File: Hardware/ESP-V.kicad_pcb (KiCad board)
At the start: 2 copper layers, 23.2 x 37.4 mm, 43 parts, among them J1 USB_C_Receptacle_USB2.0, J2 Conn_01x16_Male, J3 Conn_01x14_Female, J4 USB_A, U1 CH552E, U2 AP7333-33SRG-7, U3 AP7333-33SRG-7, U4 ESP32-C3, Y1 40MHz, Y2 32k

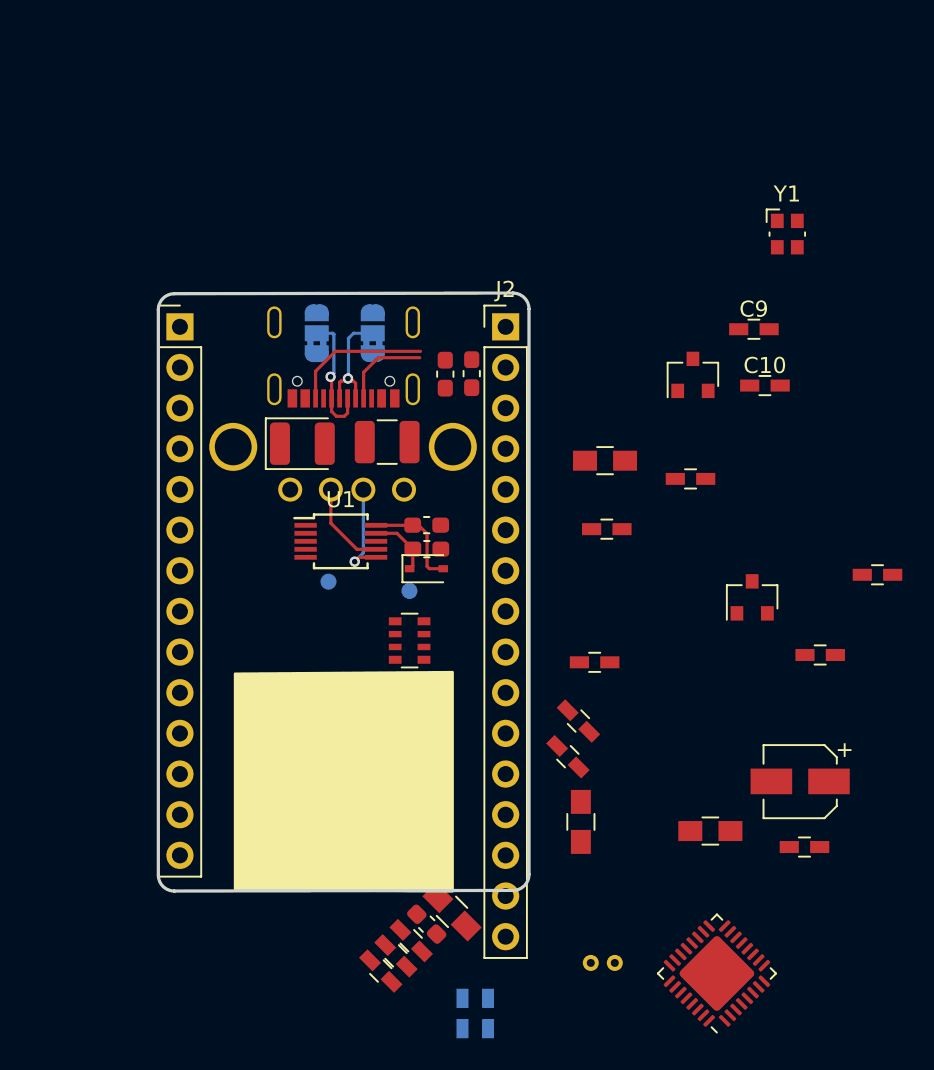
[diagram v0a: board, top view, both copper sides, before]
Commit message: v1.1 ready to order
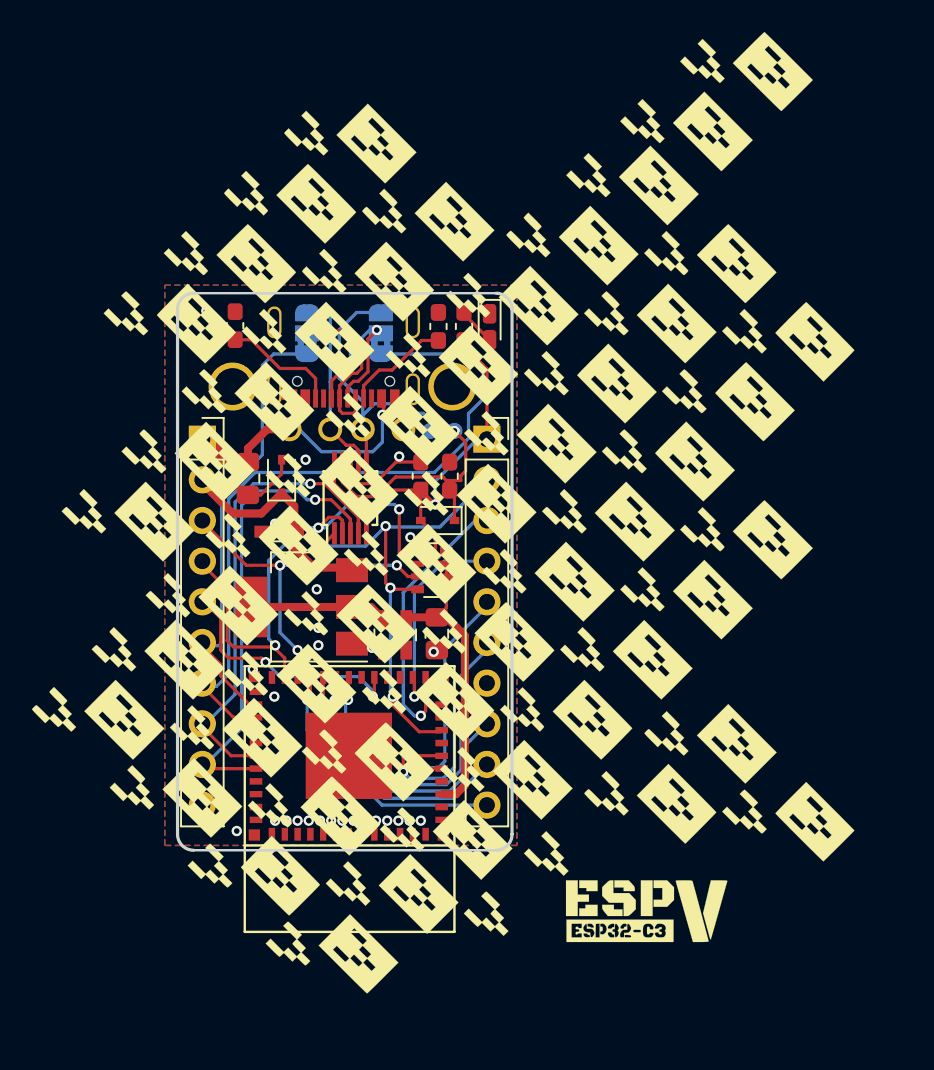
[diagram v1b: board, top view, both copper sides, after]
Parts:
- removed C1: 100uF, Capacitors_SMD:CP_Elec_4x4.5
- removed C10, C15, C18, C9: 10nF, Capacitors_SMD:C_0603_HandSoldering
- removed C11, C12: 22uF 0805, Capacitors_SMD:C_0805_HandSoldering
- removed C13, C3, C5, C8: 1uF, Capacitors_SMD:C_0603_HandSoldering
- removed C14, C2: 10uF, Capacitors_SMD:C_0805_HandSoldering
- removed C16: 100nF, Capacitors_SMD:C_0603_HandSoldering
- removed C17: 10uF, Capacitors_SMD:C_0603_HandSoldering
- removed C19: 10pF, Capacitors_SMD:C_0603_HandSoldering
- removed C24: 100nF, Capacitor_SMD:C_0603_1608Metric_Pad1.05x0.95mm_HandSolder
- removed U4: ESP32-C3, Package_DFN_QFN:QFN-32-1EP_5x5mm_P0.5mm_EP3.45x3.45mm
- removed Y1: 40MHz, Crystal:Crystal_SMD_Abracon_ABM10-4Pin_2.5x2.0mm
- removed Y2: 32k, Crystal:Crystal_DS10_D1.0mm_L4.3mm_Horizontal
- added D2: LED, LED_SMD:LED_0603_1608Metric_Castellated, F.Cu at (113.3, 78.6)
- added G***: LOGO, art and silk:frontsilk, F.Cu at (110.4, 90.2)
- added G***: LOGO, art and silk:frontv11, B.Cu at (104.3, 94.5)
- added R3: R_Small, Resistor_SMD:R_0603_1608Metric_Pad1.05x0.95mm_HandSolder, F.Cu at (111.7, 78.6)
- C20: value 1uF -> 10uF; footprint Capacitors_SMD:C_0603_HandSoldering -> Capacitor_SMD:C_0805_2012Metric_Pad1.15x1.40mm_HandSolder
- D1: footprint Diode_SMD:D_1210_3225Metric -> Diode_SMD:D_SOD-323
- J2: value Conn_01x16_Male -> Conn_01x10_Female; footprint Connector_PinHeader_2.54mm:PinHeader_1x16_P2.54mm_Vertical -> Connector_PinSocket_2.54mm:PinSocket_1x10_P2.54mm_Vertical
- J3: value Conn_01x14_Female -> Conn_01x10_Female; footprint Connector_PinHeader_2.54mm:PinHeader_1x14_P2.54mm_Vertical -> Connector_PinSocket_2.54mm:PinSocket_1x10_P2.54mm_Vertical
- L1: footprint Inductor_SMD:L_1210_3225Metric -> Inductor_SMD:L_0805_2012Metric_Pad1.15x1.40mm_HandSolder
- U2: value AP7333-33SRG-7 -> NCP1117-3.3_SOT223; footprint TO_SOT_Packages_SMD:SOT-23 -> Package_TO_SOT_SMD:SOT-223-3_TabPin2
- U3: value AP7333-33SRG-7 -> ESP32-C3-MINI-1; footprint TO_SOT_Packages_SMD:SOT-23 -> footprint:ESP32-c3-mini1
- moved C7 29.7 mm to (108.1, 97.8), turned to 270 degrees
- moved C23 29.4 mm to (106.7, 97.8), turned to 270 degrees
- moved U2 28.4 mm to (101.5, 96.1), turned to 180 degrees
- moved U3 27.1 mm to (104.5, 105.4), turned to 180 degrees
- moved C4 21.3 mm to (100.2, 91.4)
- moved R1 15.1 mm to (97.4, 78.5), turned to 270 degrees
- moved TP1 11.4 mm to (109.6, 85.1), turned to 90 degrees
- moved C20 11.2 mm to (110.0, 97.8), turned to 270 degrees
- moved TP2 10.4 mm to (111.1, 85.1)
- moved L1 8.99 mm to (98.2, 88.1), turned to 90 degrees
- moved J3 7.16 mm to (95.3, 85.6)
- moved J2 7.12 mm to (113.1, 85.6)
- moved C26 4.78 mm to (110.8, 87.9), turned to 90 degrees
- moved RN1 4.62 mm to (109.7, 93.8)
- moved JP1 4.10 mm to (101.9, 79.0)
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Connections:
- J1 pad 1: (no net) -> GND
- J1 pad A8: (no net) -> Net-(J1-PadA8)
- J1 pad B8: (no net) -> Net-(J1-PadB8)
- J2 pad 10: /GP06 -> /GP07
- J2 pad 2: +3.3VA -> /ESP_ENABLE
- J2 pad 3: /ESP_ENABLE -> /GP00
- J2 pad 4: /GP00 -> /GP01
- J2 pad 5: /GP01 -> /GP02
- J2 pad 6: /GP02 -> /GP03
- J2 pad 7: /GP03 -> /GP04
- J2 pad 8: /GP04 -> /GP05
- J2 pad 9: /GP05 -> /GP06
- J3 pad 10: /ESPUSB- -> GND
- J3 pad 3: /GP11 -> /GP08
- J3 pad 4: /GP12 -> /BLSEL
- J3 pad 5: /GP13 -> /GP10
- J3 pad 6: /GP14 -> /ESPUSB-
- J3 pad 7: /GP15 -> /ESPUSB+
- J3 pad 8: /GP16 -> /ESP_RX
- J3 pad 9: /GP17 -> /ESP_TX
- RN1 pad 1: /GP10 -> Net-(RN1-Pad1)
- RN1 pad 8: GND -> Net-(RN1-Pad8)
- U1 pad 1: (no net) -> /ESP_ENABLE
- U3 pad 2: +3.3VA -> GND
- U3 pad 3: VDD -> +3V3
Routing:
- net +3V3: track 6.53 -> 57.5 mm, vias 0 -> 1
- net /ESPUSB+: track 0.00 -> 45.3 mm
- net /BLSEL: track 0.00 -> 32.8 mm, vias 0 -> 3
- net /ESP_ENABLE: track 0.00 -> 30.4 mm, vias 0 -> 4
- net /ESP_TX: track 0.00 -> 29.6 mm, vias 0 -> 1
- net /ESP_RX: track 0.00 -> 29.0 mm, vias 0 -> 1
- net /ESPUSB-: track 0.00 -> 28.3 mm
- net VBUS: track 0.00 -> 23.0 mm, vias 0 -> 1
- net /GP08: track 0.00 -> 22.3 mm, vias 0 -> 3
- net /GP04: track 0.00 -> 18.8 mm, vias 0 -> 1
- net /GP00: track 0.00 -> 18.0 mm, vias 0 -> 1
- net /GP05: track 0.00 -> 17.6 mm, vias 0 -> 1
- net /GP07: track 0.00 -> 16.6 mm, vias 0 -> 1
- net /GP06: track 0.00 -> 16.5 mm, vias 0 -> 1
- net /GP10: track 0.00 -> 15.6 mm, vias 0 -> 2
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- added copper zone on B.Cu, net GND
- added copper zone on F.Cu, net GND
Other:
- board size 23.2 x 37.4 mm -> 20.9 x 34.8 mm
- board text removed: "V1.0"
